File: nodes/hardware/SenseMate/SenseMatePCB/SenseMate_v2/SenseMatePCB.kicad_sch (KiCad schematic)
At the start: 16 parts, among them J1 Conn_01x04, J3 Conn_Coaxial, J5 Conn_01x06_Pin, M1 Motor_DC, Q1 2SC1815, Q2 2SC1815, SW5 SW_DPDT_x2, U1 XIAO-nRF52840-Plus-SMD, U2 RFM95W-868S2

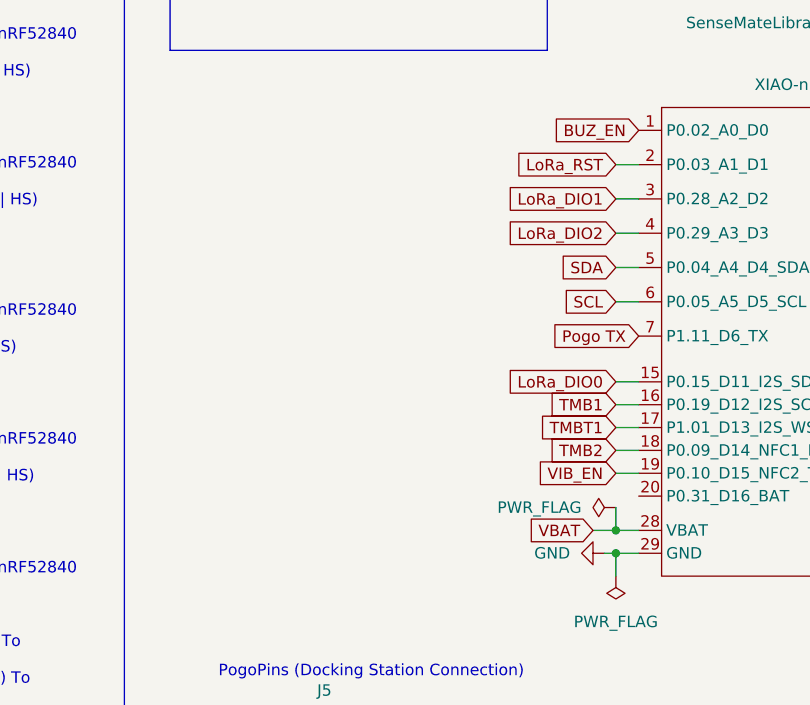
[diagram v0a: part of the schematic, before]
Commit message: castellations almost done
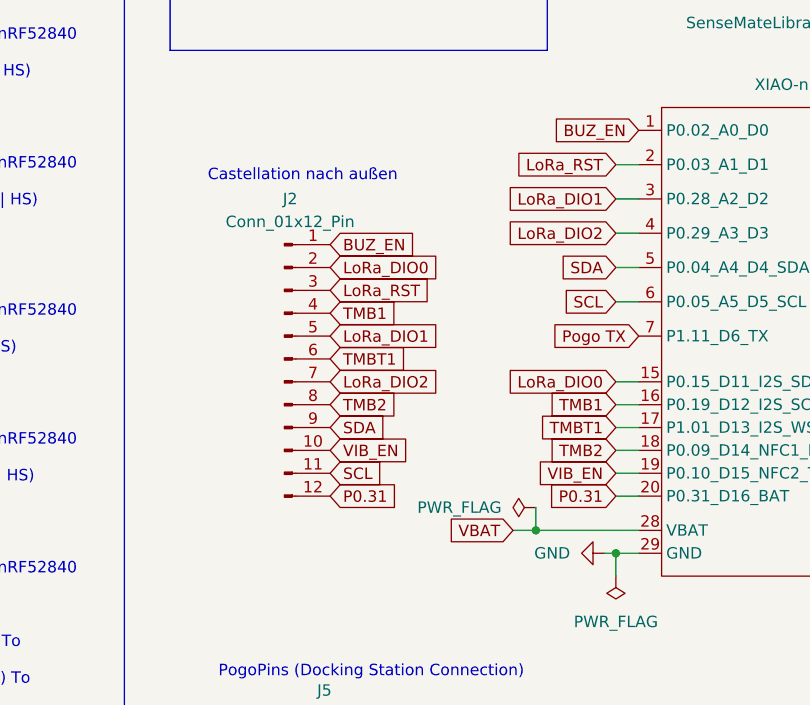
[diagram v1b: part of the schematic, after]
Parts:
- added J2: Conn_01x12_Pin, SenseMateLibrary:Castellated_1x12_2.00mm, symbol Connector:Conn_01x12_Pin
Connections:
- net BUZ_EN: now also J2.1 (Pin_1)
- net LoRa_DIO0: now also J2.2 (Pin_2)
- net LoRa_DIO1: now also J2.5 (Pin_5)
- net LoRa_DIO2: now also J2.7 (Pin_7)
- net LoRa_RST: now also J2.3 (Pin_3)
- net SCL: now also J2.11 (Pin_11)
- net SDA: now also J2.9 (Pin_9)
- net TMB1: now also J2.4 (Pin_4)
- net TMB2: now also J2.8 (Pin_8)
- net TMBT1: now also J2.6 (Pin_6)
- net VIB_EN: now also J2.10 (Pin_10)
- net P0.31: now reaches U1.20 (P0.31_D16_BAT)
- net P0.31: now also J2.12 (Pin_12)
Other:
- note added: "Castellation nach außen"

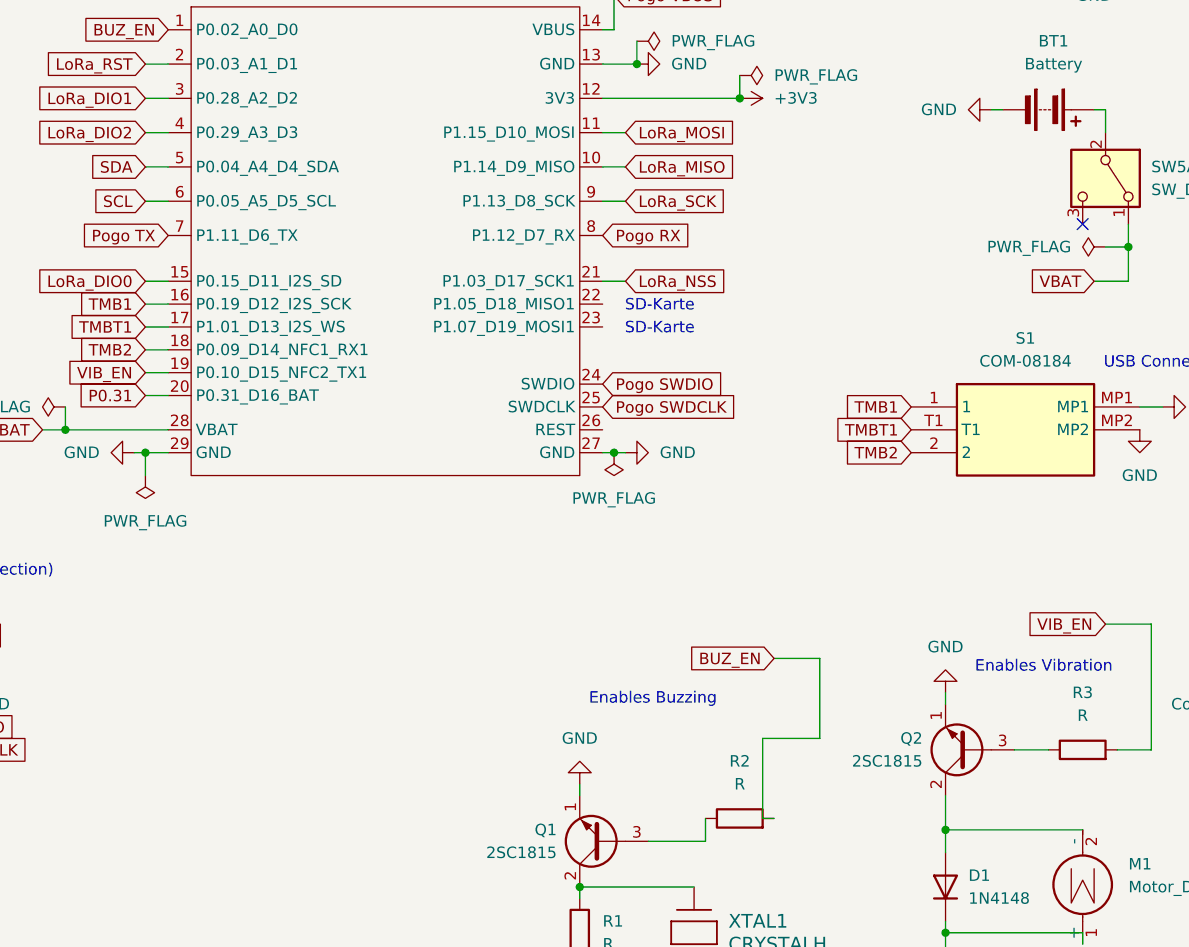
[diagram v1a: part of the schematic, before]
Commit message: SENSEMATE V3 DONE
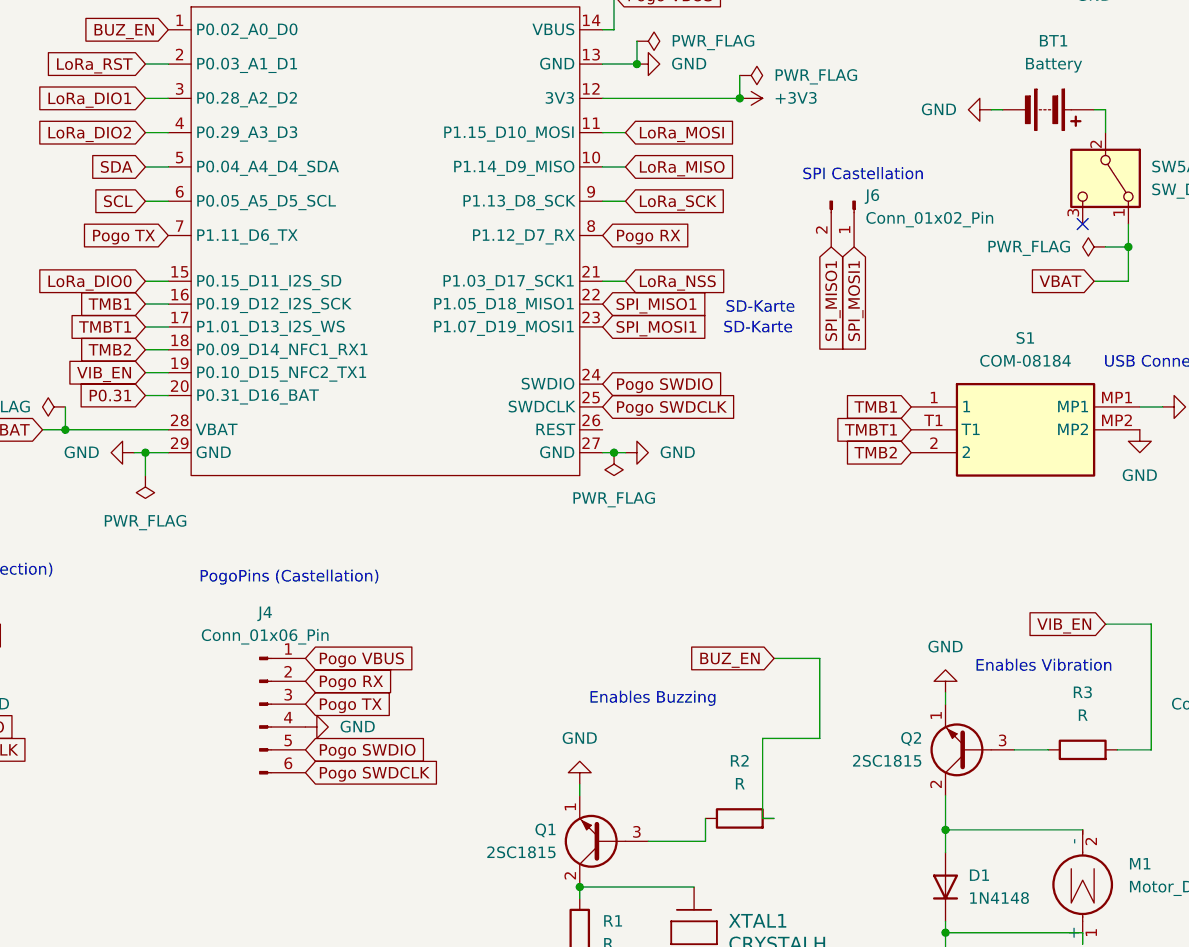
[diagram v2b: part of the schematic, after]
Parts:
- added J4: Conn_01x06_Pin, SenseMateLibrary:Castellated_1x6_2.00mm, symbol Connector:Conn_01x06_Pin
- added J6: Conn_01x02_Pin, SenseMateLibrary:Castellated_1x2_2.00mm, symbol Connector:Conn_01x02_Pin
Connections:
- net GND: now also J4.4 (Pin_4)
- net Pogo RX: now also J4.2 (Pin_2)
- net Pogo SWDCLK: now also J4.6 (Pin_6)
- net Pogo SWDIO: now also J4.5 (Pin_5)
- net Pogo TX: now also J4.3 (Pin_3)
- net Pogo VBUS: now also J4.1 (Pin_1)
- net SPI_MISO1: now reaches U1.22 (P1.05_D18_MISO1)
- net SPI_MISO1: now also J6.2 (Pin_2)
- net SPI_MOSI1: now reaches U1.23 (P1.07_D19_MOSI1)
- net SPI_MOSI1: now also J6.1 (Pin_1)
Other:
- note added: "PogoPins (Castellation)"
- note added: "SPI Castellation"
